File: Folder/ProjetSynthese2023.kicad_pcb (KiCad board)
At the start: 2 copper layers, 198.1 x 129.5 mm, 21 parts

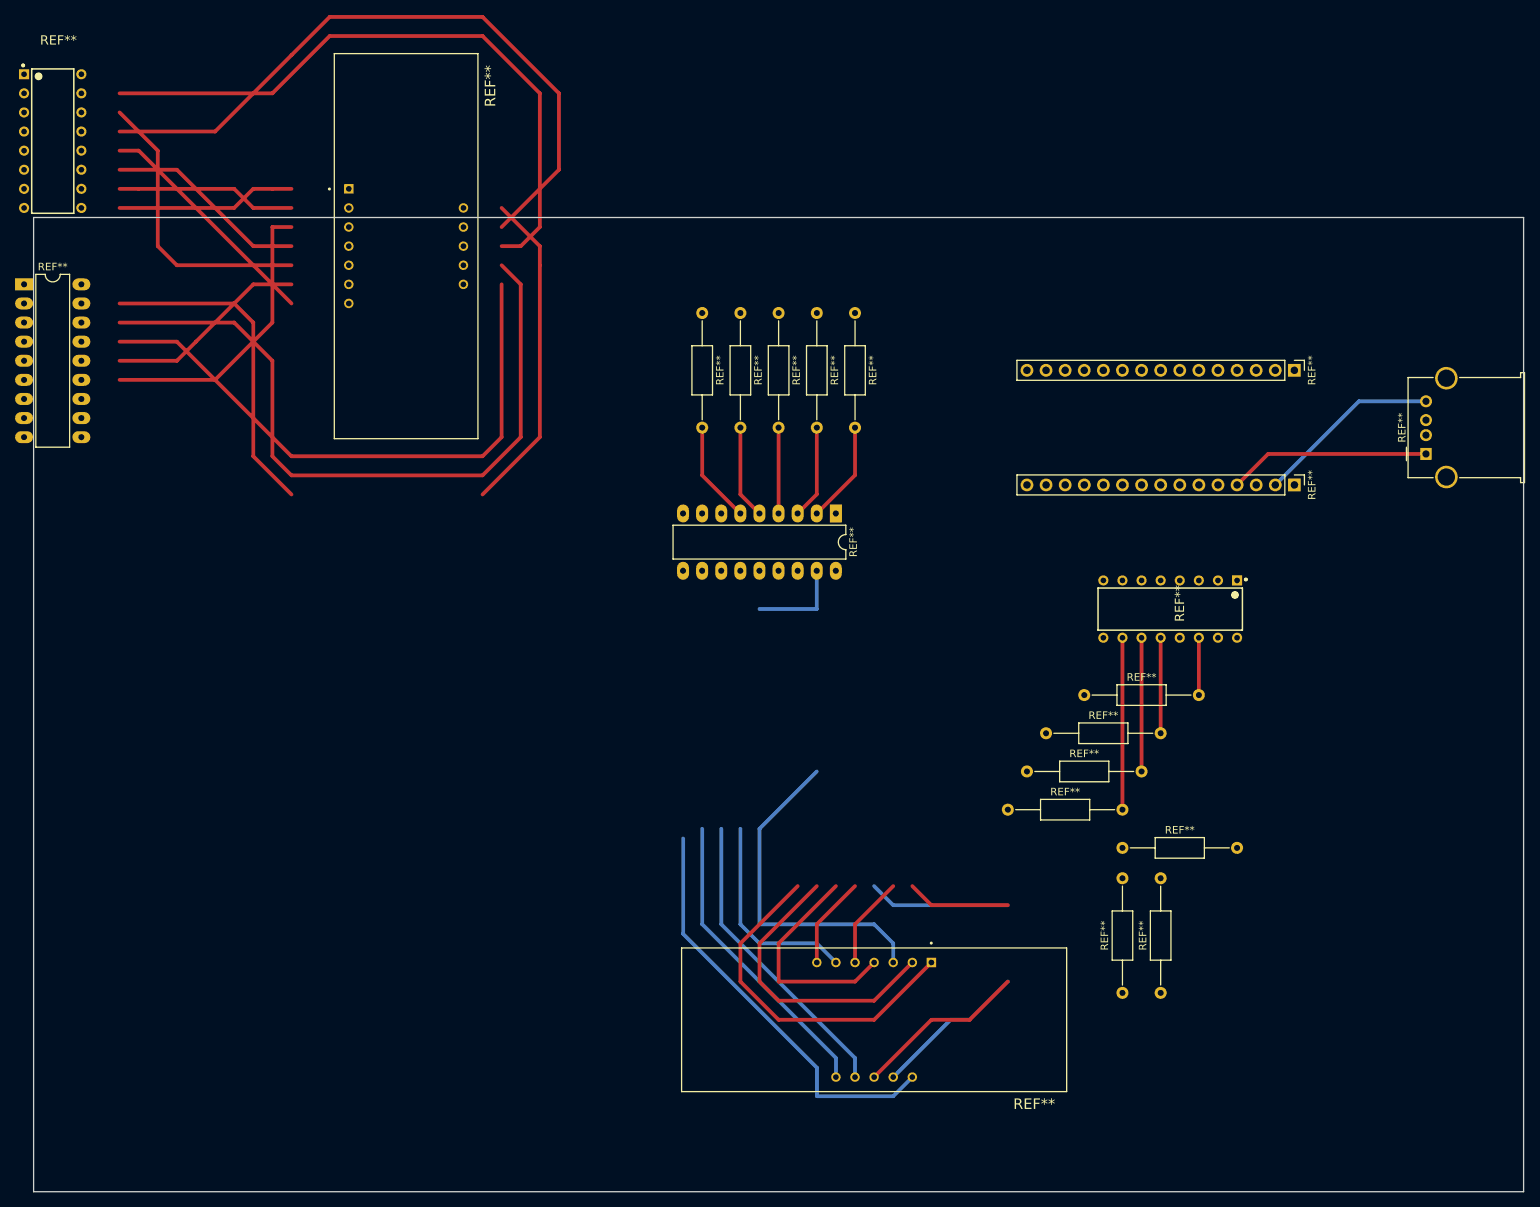
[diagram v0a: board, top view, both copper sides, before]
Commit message: ok
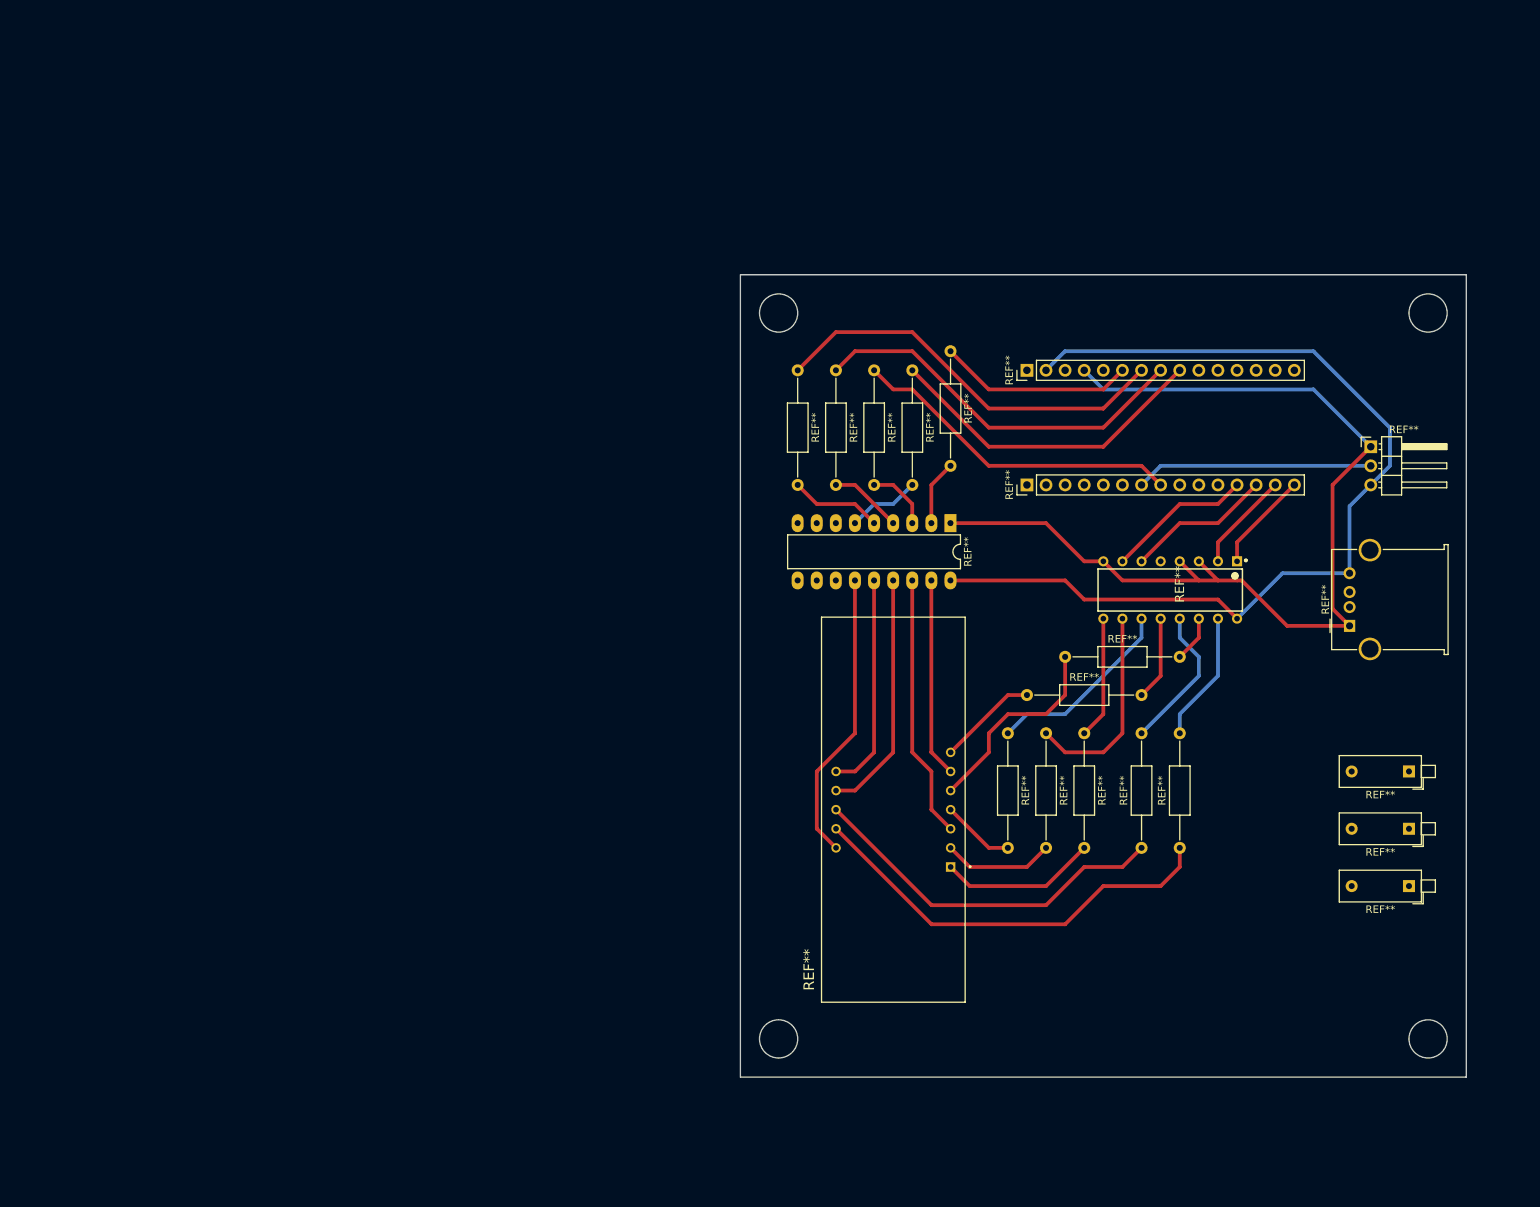
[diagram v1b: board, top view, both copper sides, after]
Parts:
- removed the REF** at (34.3, 21.6)
- removed the REF** at (38.1, 2.54)
- removed the REF** at (85.1, 16.5)
- added REF**: SW_DIP_SPSTx01_Piano_10.8x4.1mm_W7.62mm_P2.54mm, Button_Switch_THT:SW_DIP_SPSTx01_Piano_10.8x4.1mm_W7.62mm_P2.54mm, F.Cu at (218.4, 86.4)
- added REF**: PinHeader_1x03_P2.54mm_Horizontal, Connector_PinHeader_2.54mm:PinHeader_1x03_P2.54mm_Horizontal, F.Cu at (213.4, 43.2)
- added REF**: SW_DIP_SPSTx01_Piano_10.8x4.1mm_W7.62mm_P2.54mm, Button_Switch_THT:SW_DIP_SPSTx01_Piano_10.8x4.1mm_W7.62mm_P2.54mm, F.Cu at (218.4, 101.6)
- added REF**: SW_DIP_SPSTx01_Piano_10.8x4.1mm_W7.62mm_P2.54mm, Button_Switch_THT:SW_DIP_SPSTx01_Piano_10.8x4.1mm_W7.62mm_P2.54mm, F.Cu at (218.4, 94.0)
- moved REF** 38.7 mm to (167.6, 33.0), turned to 90 degrees
- moved REF** 38.7 mm to (167.6, 48.3), turned to 90 degrees
- moved REF** 28.1 mm to (149.9, 91.4), turned to 90 degrees
- moved REF** 25.0 mm to (210.5, 67.0)
- moved REF** 21.6 mm to (165.1, 81.3), turned to -90 degrees
- moved REF** 19.4 mm to (188.0, 96.5)
- moved REF** 19.4 mm to (182.9, 96.5)
- moved REF** 19.3 mm to (142.2, 33.0)
- moved REF** 19.3 mm to (152.4, 33.0)
- moved REF** 18.5 mm to (157.5, 30.5)
- moved REF** 15.5 mm to (167.6, 76.2)
- moved REF** 15.3 mm to (157.5, 53.3)
- moved REF** 10.8 mm to (137.2, 33.0)
- moved REF** 8.03 mm to (147.3, 33.0)
- moved REF** 5.68 mm to (170.2, 81.3), turned to -90 degrees
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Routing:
- net (no net): track 1260.6 -> 1108.5 mm
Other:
- board size 198.1 x 129.5 mm -> 96.5 x 106.7 mm
